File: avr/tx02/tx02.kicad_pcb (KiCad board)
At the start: 2 copper layers, 21.6 x 7.6 mm, 16 parts, among them J1 USB-C, J2 OUT, SW1 SW_Push, SW2 SW_SPDT, U1 ATtiny202-SS, U2 CH340E

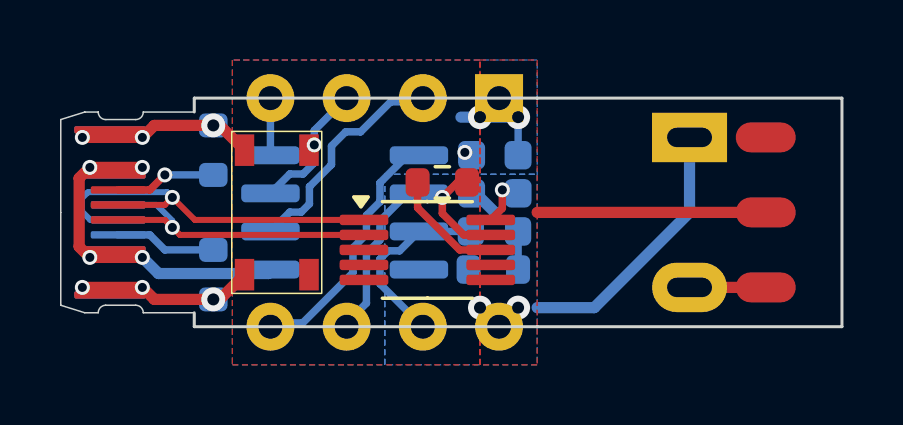
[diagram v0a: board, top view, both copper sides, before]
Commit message: -
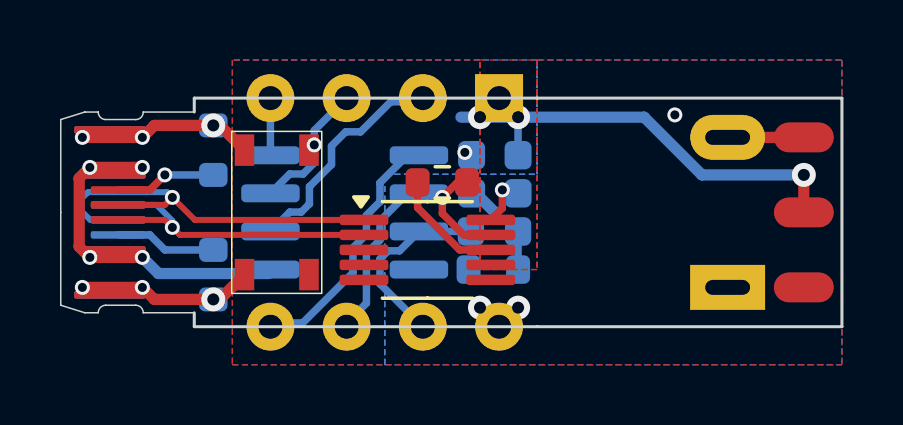
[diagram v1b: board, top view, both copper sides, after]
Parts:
- moved C2 1.27 mm to (116.5, 100.0), turned to 0 degrees
- moved SW2 1.27 mm to (119.0, 100.0), turned to 180 degrees
- moved G*** 0.69 mm to (112.8, 100.0)
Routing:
- net GND: track 23.0 -> 14.1 mm, vias 9 -> 10
- net VCC: track 22.2 -> 26.2 mm, vias 6 -> 7
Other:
- board text added: "on off"
